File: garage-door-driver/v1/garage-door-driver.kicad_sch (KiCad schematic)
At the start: 5 parts, among them J1 Screw_Terminal_01x02, J2 Conn_01x07_Pin, J3 Screw_Terminal_01x02, U1 WeMos_D1_mini, U2 4N35

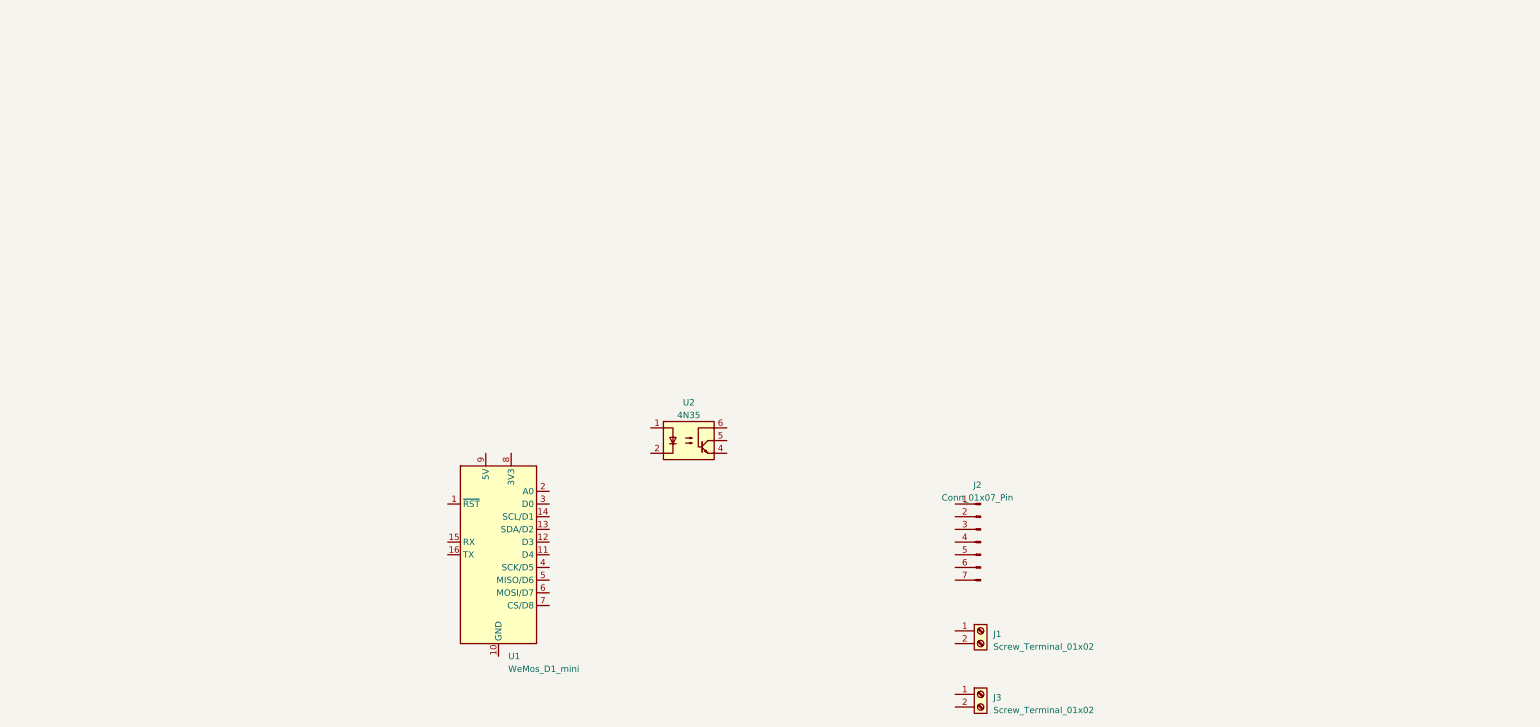
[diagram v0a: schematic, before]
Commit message: sch
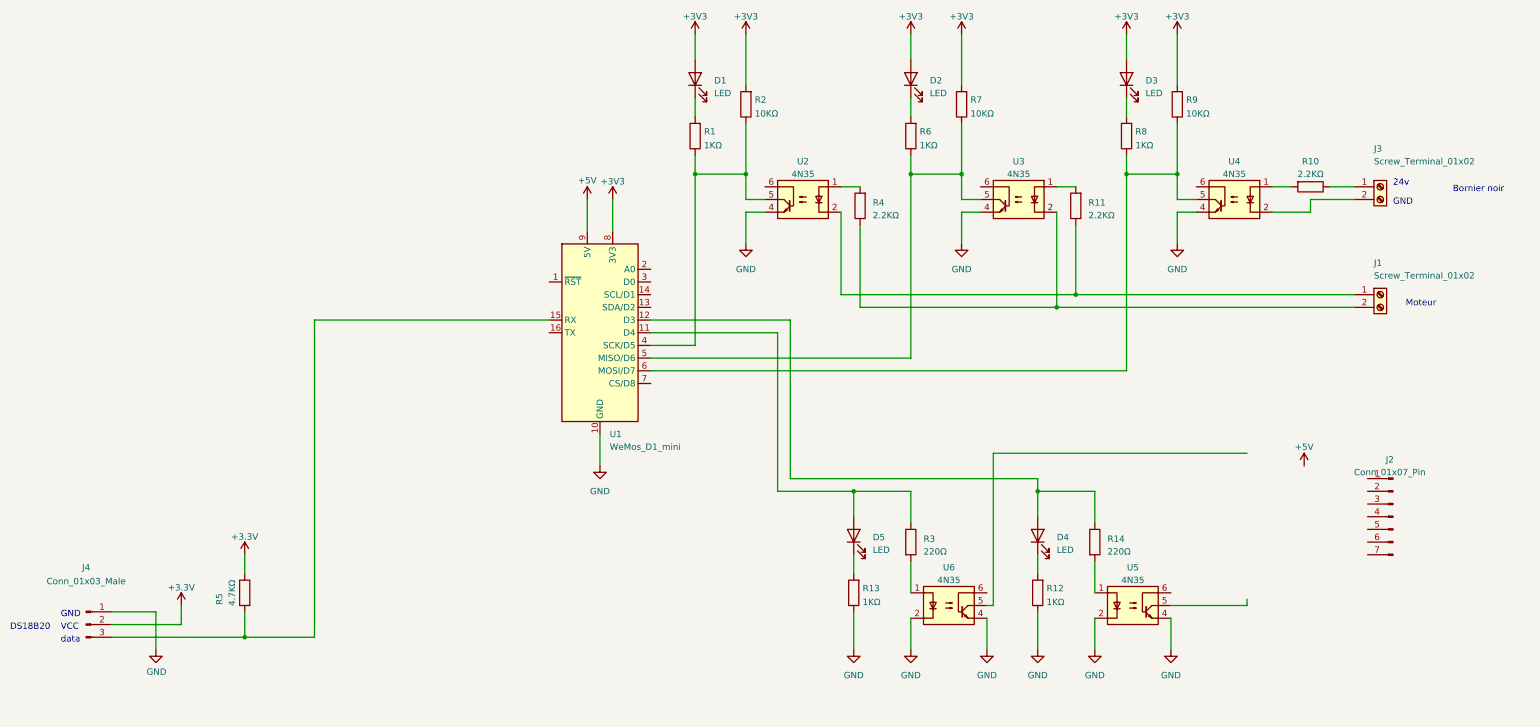
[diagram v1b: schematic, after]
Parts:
- added D1, D2, D3, D4, D5: LED, Diode_SMD:D_0805_2012Metric, symbol Device:LED
- added J4: Conn_01x03_Male, Connector_PinHeader_2.54mm:PinHeader_1x03_P2.54mm_Vertical, symbol Connector:Conn_01x03_Male
- added R1, R12, R13, R6, R8: 1KΩ, Resistor_SMD:R_0603_1608Metric, symbol Device:R
- added R10, R11, R4: 2.2KΩ, Resistor_SMD:R_0603_1608Metric, symbol Device:R
- added R14, R3: 220Ω, Resistor_SMD:R_0603_1608Metric, symbol Device:R
- added R2, R7, R9: 10KΩ, Resistor_SMD:R_0603_1608Metric, symbol Device:R
- added R5: 4.7KΩ, Resistor_SMD:R_0402_1005Metric, symbol Device:R
- added U3, U4, U5, U6: 4N35, Package_DIP:DIP-6_W7.62mm, symbol Isolator:4N35
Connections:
- net at J3.1 (Pin_1): now also R10.1
- net at J3.2 (Pin_2): now also U4.2
- net at U2.1: now also R4.2
- net at U2.2: now also J1.1 (Pin_1), R11.1
- net GND: now reaches U2.4
- net GND: now also U1.10 (GND), J4.1 (Pin_1), R12.1, R13.1, U3.4, U4.4, U5.2, U5.4, U6.2, U6.4
- net at U2.5: now also U1.4 (SCK/D5), R1.1, R2.1
- net at J1.2 (Pin_2): now also R4.1, U3.2
- net at U1.11 (D4): now also D5.2 (A), R3.1
- net at U1.12 (D3): now also D4.2 (A), R14.1
- net at U1.15 (RX): now also J4.3 (Pin_3), R5.2
- net at U1.5 (MISO/D6): now also R6.1, R7.1, U3.5
- net at U1.6 (MOSI/D7): now also R8.1, R9.1, U4.5
- net +3V3: now reaches U1.8 (3V3)
- net +3V3: now also D1.2 (A), D2.2 (A), D3.2 (A), J4.2 (Pin_2), R2.2, R5.1, R7.2, R9.2
- net +5V: now reaches U1.9 (5V)
- new net: R3.2, U6.1
- new net: R11.2, U3.1
- new net: D1.1 (K), R1.2
- new net: D3.1 (K), R8.2
- new net: D2.1 (K), R6.2
- new net: D5.1 (K), R13.2
- new net: R10.2, U4.1
- new net: D4.1 (K), R12.2
- new net: R14.2, U5.1
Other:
- note added: "24v"
- note added: "Bornier noir"
- note added: "DS18B20"
- note added: "GND"
- note added: "Moteur"
- note added: "VCC"
- note added: "data"
- moved on the sheet: J1, J2, J3, U1, U2
